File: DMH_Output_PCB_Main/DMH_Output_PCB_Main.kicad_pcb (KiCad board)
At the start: 2 copper layers, 49 x 175 mm, 92 parts, among them J0 Conn_01x01, J1 TRS_Jack_6.35mm_Sw, J100 IDC_02x05, J2 TRS_Jack_6.35mm_Sw, J200 IDC_02x05, J23 Conn_01x06, J24 Conn_01x02, J25 Conn_01x02, J26 Conn_01x06_PinHeader, J27 Conn_01x06_PinHeader, J28 Conn_01x06, J29 Conn_01x04_PinHeader, J3 TRS_Jack_6.35mm_Sw, J31 Conn_01x06_PinHeader, J35 Conn_01x02_PinHeader, J36 Conn_01x02_PinHeader, J4 TRS_Jack_6.35mm_Sw, J5 TRS_Jack_6.35mm_Sw, J6 TRS_Jack_6.35mm_Sw, J7 TRS_Jack_6.35mm_Sw, J8 TRS_Jack_6.35mm_Sw, J9 TRS_Jack_6.35mm_Sw, U1 TL072, U11 TL074, U13 NE5532, U15 NE5532, U20 TL072, U8 TL074

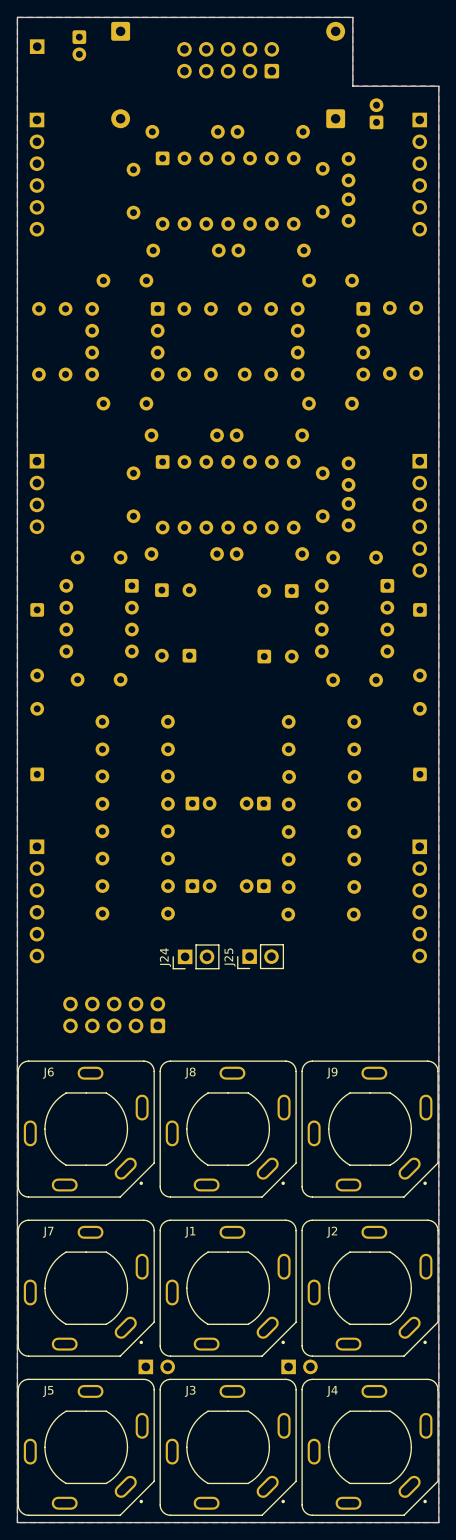
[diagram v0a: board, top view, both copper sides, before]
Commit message: Main PCB routing in progress
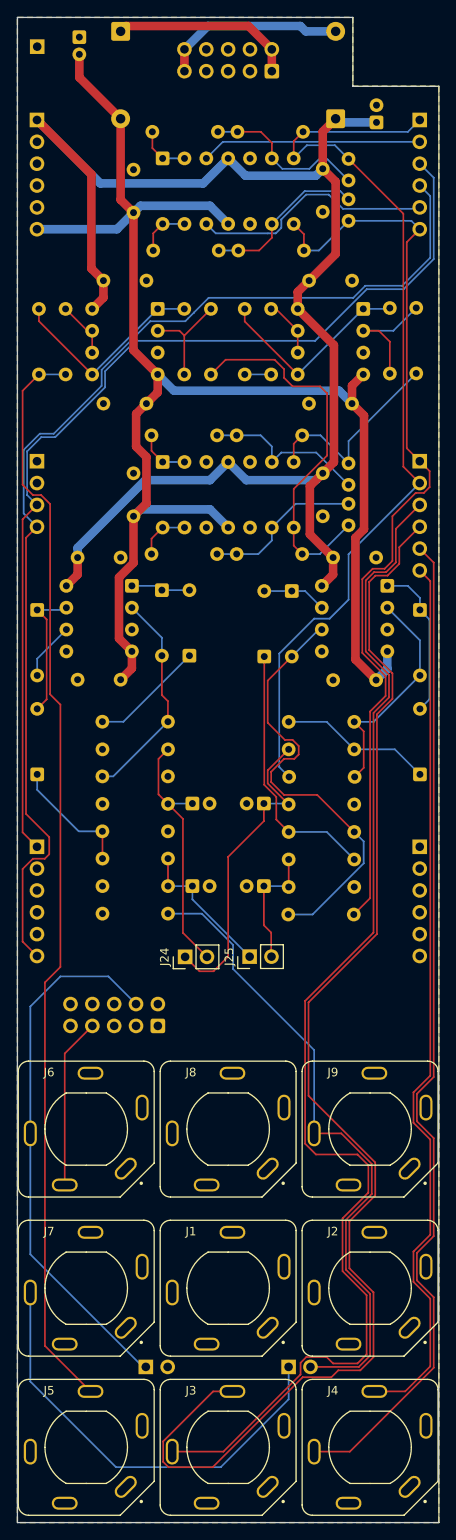
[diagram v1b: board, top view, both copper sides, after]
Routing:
- net -12V: track 0.00 -> 182.9 mm
- net +12V: track 0.00 -> 170.0 mm
- net /Balanced Line Driver/L_Bal_OUT_N_M: track 0.00 -> 153.4 mm
- net /Balanced Line Driver/L_Bal_OUT_P_M: track 0.00 -> 144.3 mm
- net /Gain Trimmer/R_Gain_IN_M: track 0.00 -> 130.4 mm
- net /Headphone Amplifier/R_HP_OUT_M: track 0.00 -> 127.4 mm
- net /Gain Trimmer/L_Gain_IN_M: track 0.00 -> 117.2 mm
- net /Balanced Line Driver/R_Bal_OUT_P_M: track 0.00 -> 117.1 mm
- net /Balanced Line Driver/L_Ch_OUT_M: track 0.00 -> 108.9 mm
- net /Balanced Line Driver/R_Ch_OUT_M: track 0.00 -> 107.5 mm
- net /Balanced Line Driver/R_Bal_OUT_N_M: track 0.00 -> 104.0 mm
- net /Input Meter/R_Ext_Meter_M: track 0.00 -> 75.2 mm
- net /PreAmp/L_Ext_IN_M: track 0.00 -> 62.7 mm
- net Net-(D5-A): track 0.00 -> 52.0 mm
- net /PreAmp/R_Ext_IN_M: track 0.00 -> 51.5 mm
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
